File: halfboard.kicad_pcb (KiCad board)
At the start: 2 copper layers, 240.1 x 87.9 mm, 54 parts, among them U1 

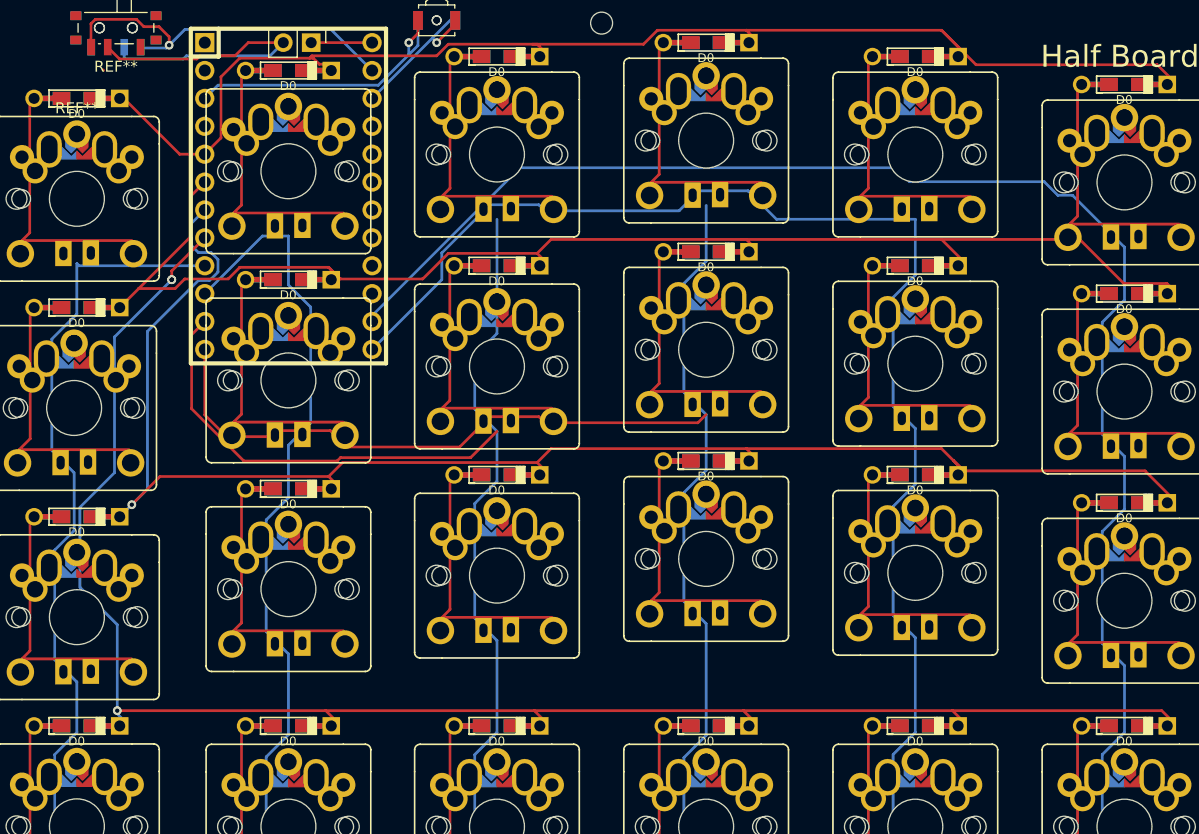
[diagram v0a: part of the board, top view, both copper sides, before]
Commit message: clean footprint
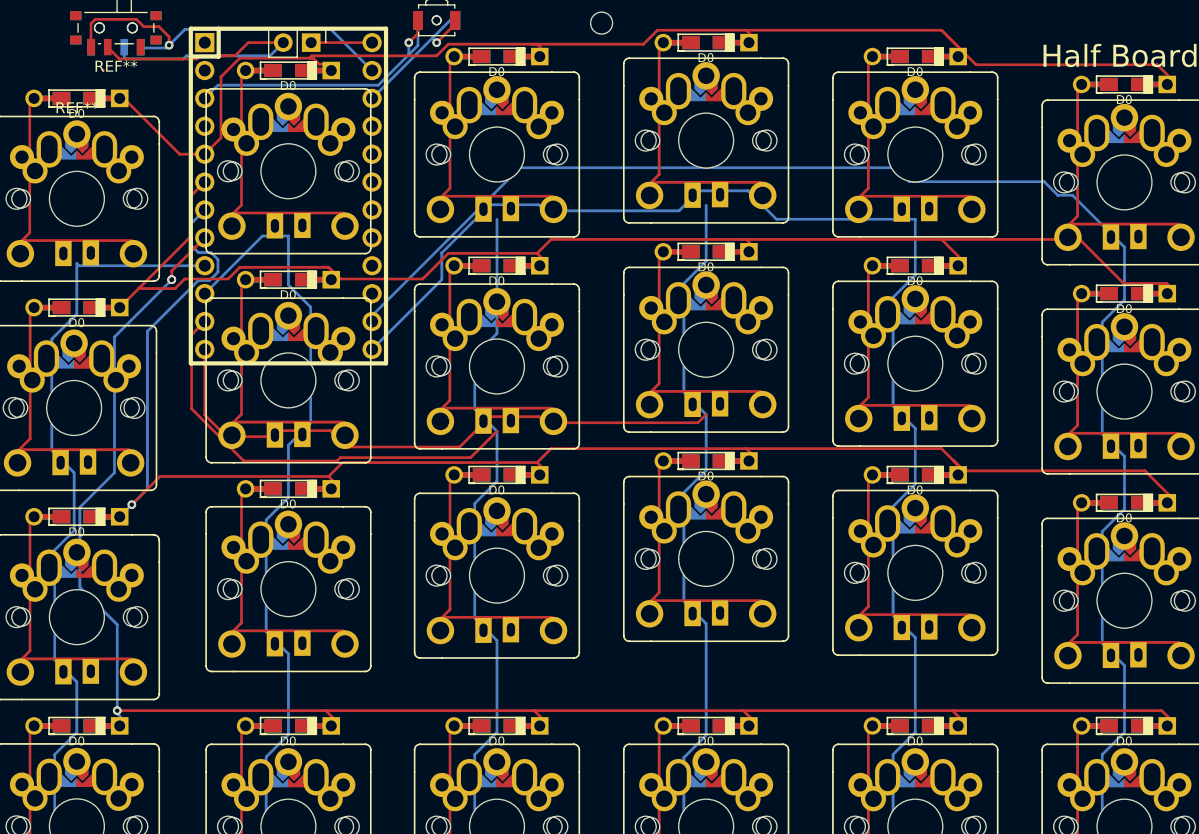
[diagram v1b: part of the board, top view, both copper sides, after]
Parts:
- removed the REF** at (52.6, 48.5) (x2)
- added REF**: SW_SPDT_PCM12, Button_Switch_SMD:SW_SPDT_PCM12, F.Cu at (52.6, 48.5)
- added REF**: SW_SPDT_PCM12, Button_Switch_SMD:SW_SPDT_PCM12, B.Cu at (52.6, 48.5)
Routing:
- net col2: track 105.6 -> 39.3 mm
- net (no net): track 0.00 -> 66.2 mm
